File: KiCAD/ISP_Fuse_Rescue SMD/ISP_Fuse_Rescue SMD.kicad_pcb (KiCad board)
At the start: 2 copper layers, 54 parts, among them Q1 MMBT3904, Q2 MMBT3904, Q5 IRF7389PbF, SW1 Reset, SW2 SW_DPDT_x2, U1 74HCT4053N, U2 74HCT4053N, U3 MC34063AP, U4 ATmega328P-PU, Y1 16MHz

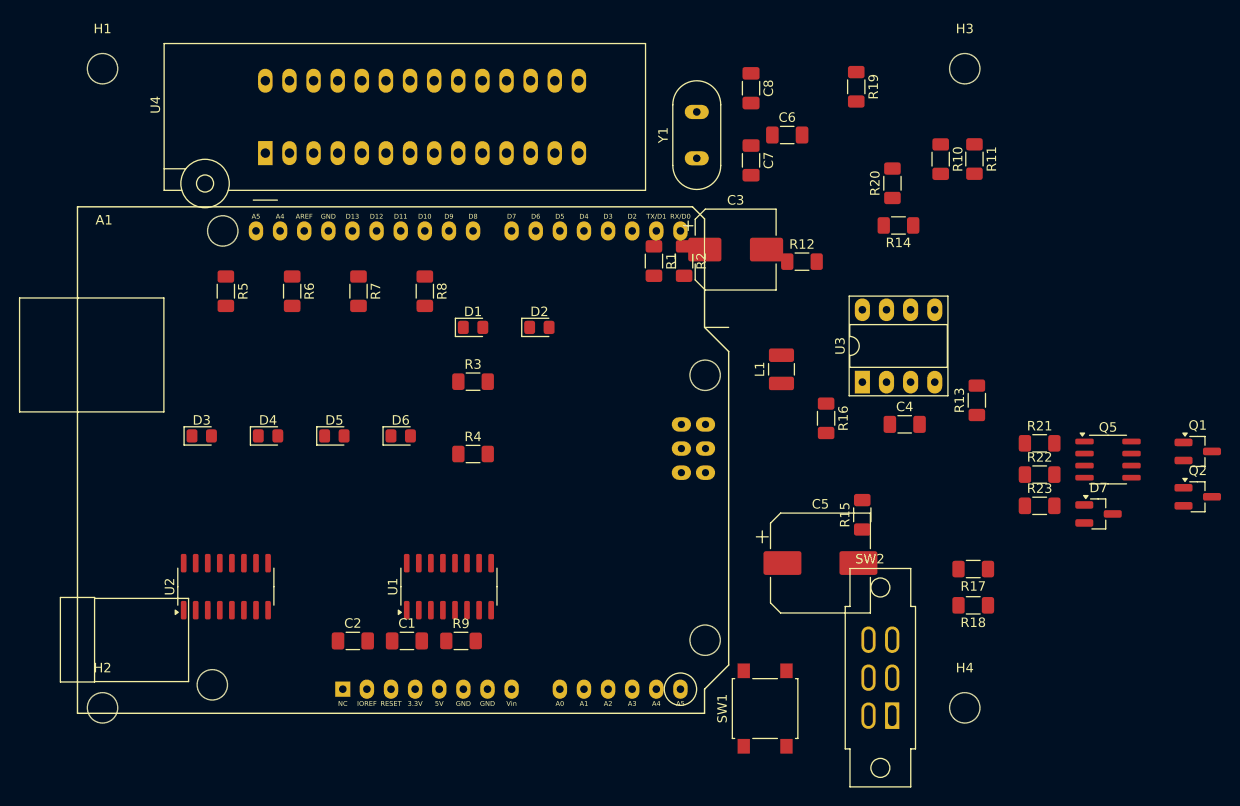
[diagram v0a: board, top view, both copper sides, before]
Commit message: smd fuse rescue
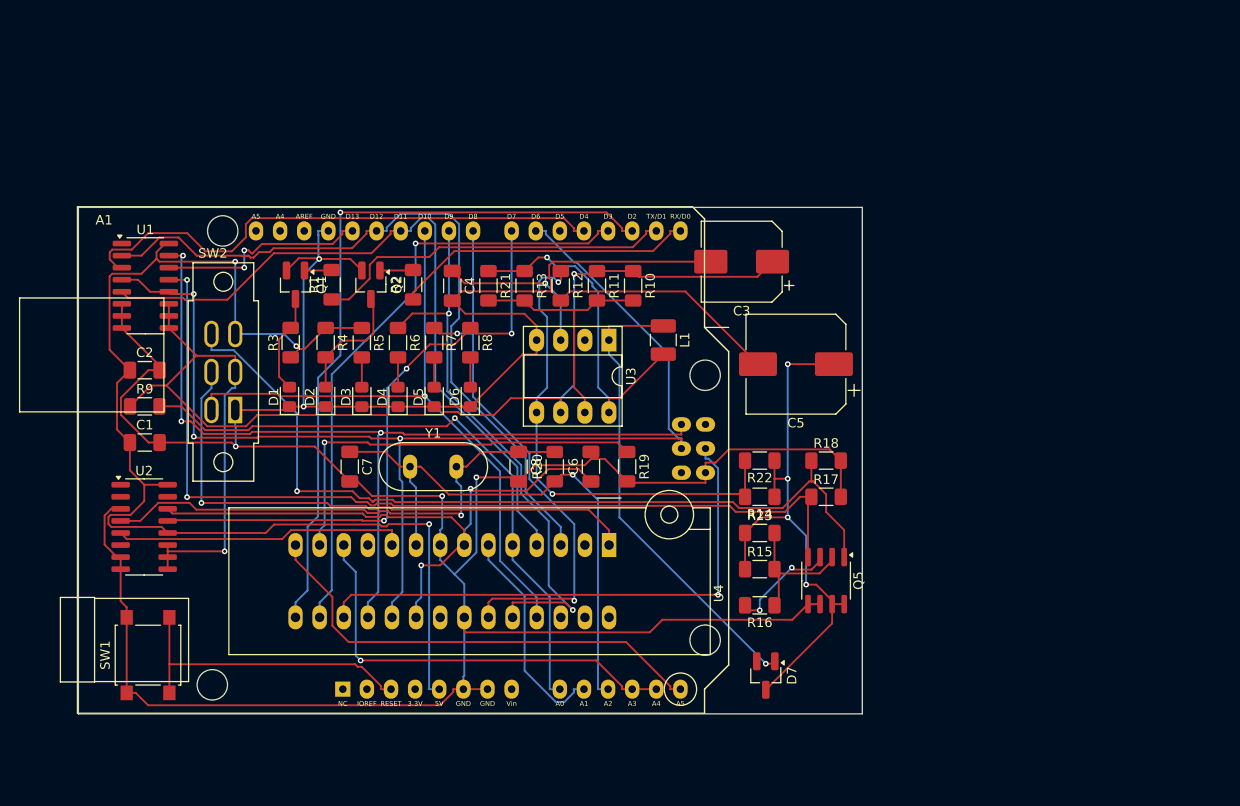
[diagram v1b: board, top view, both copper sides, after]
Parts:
- removed H1, H2, H3, H4: MountingHole, MountingHole:MountingHole_3.2mm_M3
- moved Q1 96.6 mm to (126.4, 93.2), turned to -90 degrees
- moved Q2 89.9 mm to (134.3, 93.2), turned to -90 degrees
- moved SW2 76.3 mm to (118.8, 102.4)
- moved SW1 65.2 mm to (110.8, 132.2)
- moved R21 60.4 mm to (146.7, 93.3), turned to -90 degrees
- moved U4 54.9 mm to (159.4, 120.7), turned to -90 degrees
- moved C7 53.2 mm to (132.1, 112.4)
- moved C4 49.8 mm to (142.9, 93.3), turned to -90 degrees
- moved R13 49.1 mm to (150.5, 93.3), turned to -90 degrees
- moved C8 46.8 mm to (149.9, 112.4)
- moved R19 46.7 mm to (161.3, 112.4)
- moved R20 46.4 mm to (153.7, 112.4)
- moved U1 45.0 mm to (110.6, 93.3), turned to 0 degrees
- moved Y1 44.3 mm to (138.4, 112.4), turned to 0 degrees
- moved R11 41.9 mm to (158.1, 93.3)
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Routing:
- net GND: track 0.00 -> 372.5 mm, vias 0 -> 5
- net A: track 0.00 -> 133.1 mm, vias 0 -> 2
- net +5V: track 0.00 -> 127.4 mm, vias 0 -> 3
- net SCK/TG D5: track 0.00 -> 125.5 mm, vias 0 -> 3
- net B: track 0.00 -> 98.5 mm, vias 0 -> 2
- net MISO/TG D4: track 0.00 -> 93.5 mm, vias 0 -> 3
- net Net-(Q5A-S): track 0.00 -> 89.6 mm, vias 0 -> 1
- net MISO/RDY#BSY: track 0.00 -> 78.9 mm
- net TG D1: track 0.00 -> 76.3 mm, vias 0 -> 1
- net MOSI/#OE: track 0.00 -> 75.7 mm
- net Reset/BS2: track 0.00 -> 69.9 mm, vias 0 -> 1
- net #WR: track 0.00 -> 66.4 mm, vias 0 -> 1
- net AVCC: track 0.00 -> 65.7 mm, vias 0 -> 2
- net TG D2: track 0.00 -> 64.6 mm, vias 0 -> 1
- net TG VCC: track 0.00 -> 63.8 mm, vias 0 -> 3
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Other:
- board outline added: 82.6 x 53.3 mm
